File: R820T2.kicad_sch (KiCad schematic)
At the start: 28 parts, among them U7 R820T2

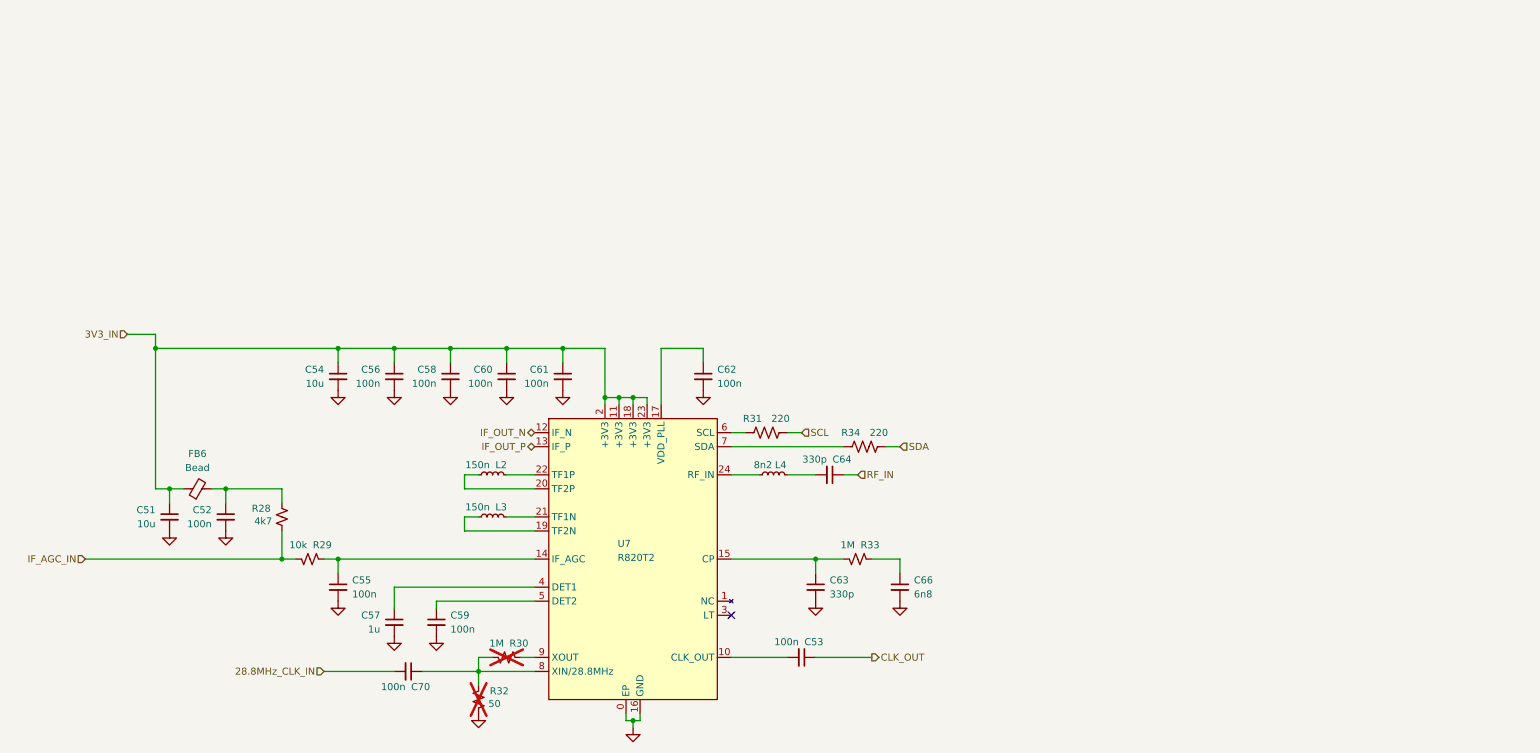
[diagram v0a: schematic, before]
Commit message: Schematic progress
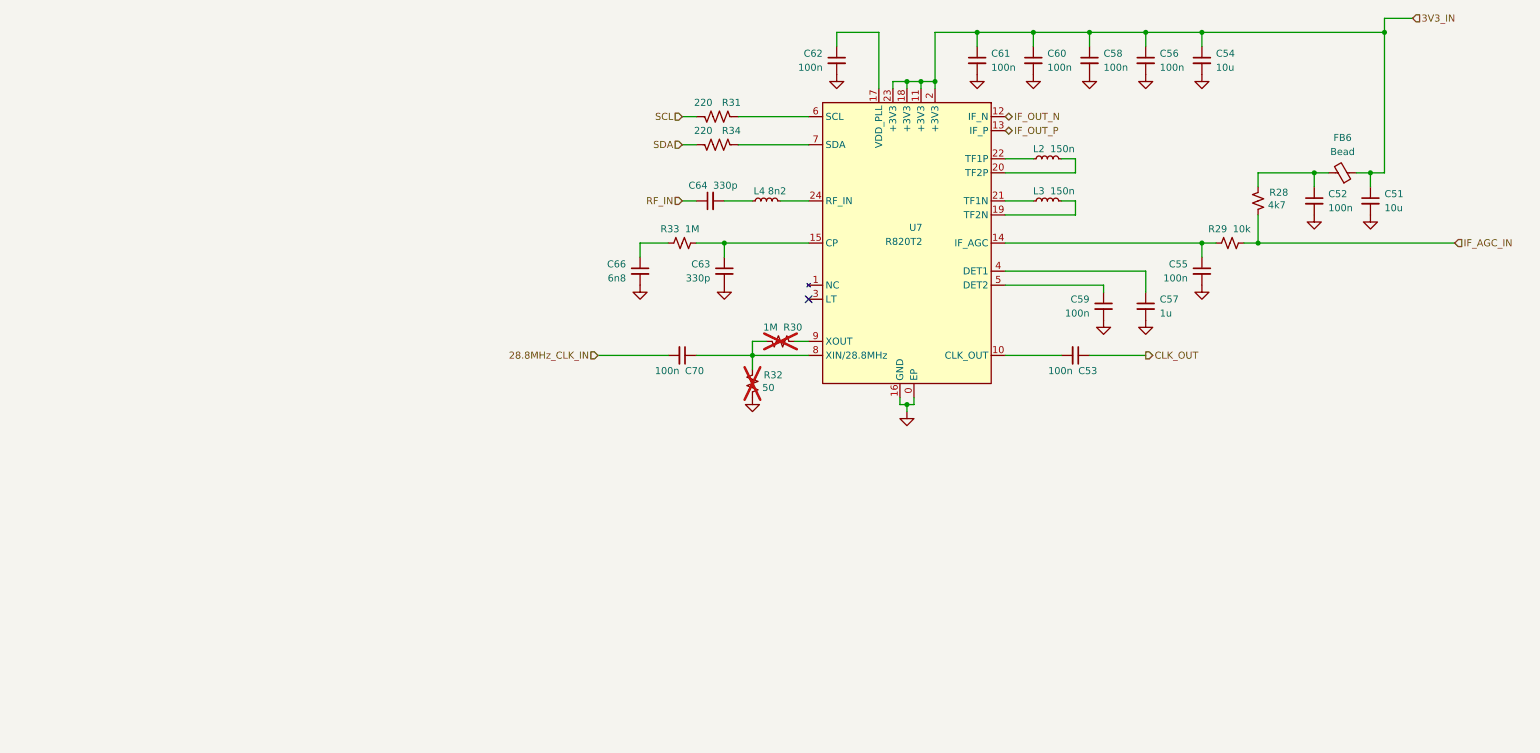
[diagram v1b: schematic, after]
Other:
- moved on the sheet: C51, C52, C53, C54, C55, C56, C57, C58, C59, C60, C61, C62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
